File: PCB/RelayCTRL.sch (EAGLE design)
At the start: 20 parts, among them Q2 BC848 30V 100mA, Q3 IRLML6402, U1 SN74HC4066D

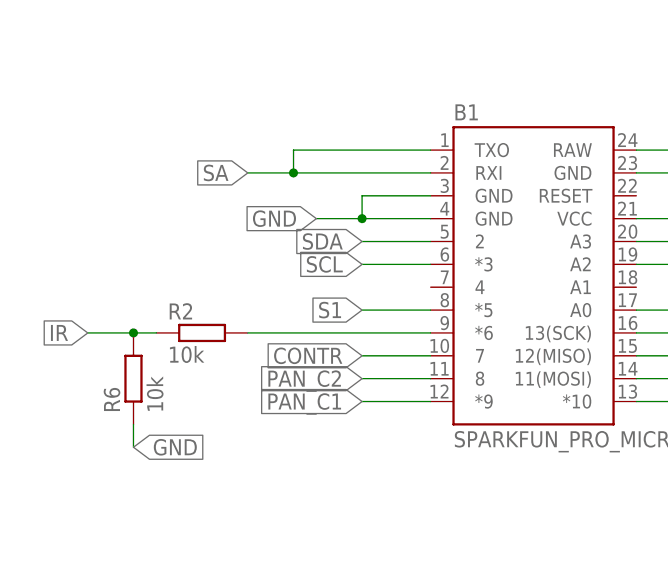
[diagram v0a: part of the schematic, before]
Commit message: fixed pcb error
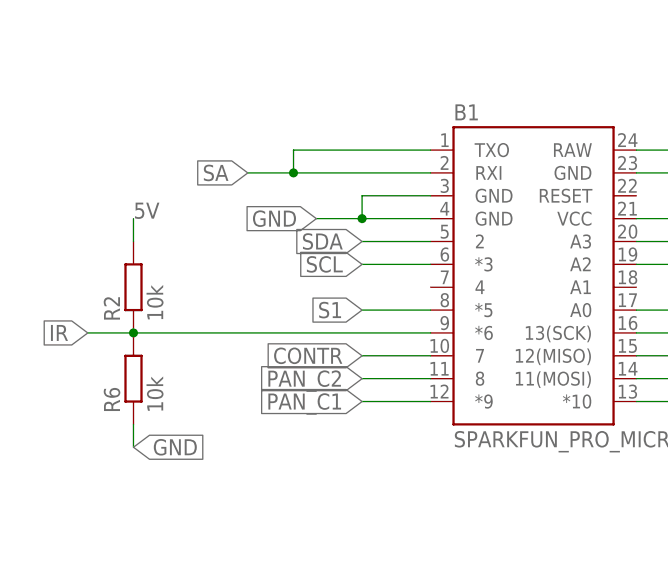
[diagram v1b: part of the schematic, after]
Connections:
- removed net N$1: B1.*6, R2.2
- net 5V: now also R2.2
- net IR: now also B1.*6
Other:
- moved on the sheet: R2
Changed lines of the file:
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@@
 <attribute name="TP_SIGNAL_NAME" x="95.25" y="-39.37" size="1.778" layer="97" rot="R180"/>
 </instance>
-<instance part="R2" gate="G$1" x="30.48" y="20.32" smashed="yes">
-<attribute name="NAME" x="26.67" y="21.8186" size="1.778" layer="95"/>
-<attribute name="VALUE" x="26.67" y="17.018" size="1.778" layer="96"/>
+<instance part="R2" gate="G$1" x="22.86" y="25.4" smashed="yes" rot="R90">
+<attribute name="NAME" x="21.3614" y="21.59" size="1.778" layer="95" rot="R90"/>
+<attribute name="VALUE" x="26.162" y="21.59" size="1.778" layer="96" rot="R90"/>
 </instance>
 <instance part="R6" gate="G$1" x="22.86" y="15.24" smashed="yes" rot="R90">
@@
 <wire x1="88.9" y1="-38.1" x2="88.9" y2="-33.02" width="0.1524" layer="91"/>
 <label x="88.9" y="-33.02" size="1.778" layer="95" rot="R90" xref="yes"/>
+</segment>
+<segment>
+<pinref part="R2" gate="G$1" pin="2"/>
+<wire x1="22.86" y1="30.48" x2="22.86" y2="33.02" width="0.1524" layer="91"/>
+<label x="22.86" y="33.02" size="1.778" layer="95"/>
 </segment>
 </net>
@@
 </segment>
 </net>
-<net name="N$1" class="0">
-<segment>
-<pinref part="B1" gate="G$1" pin="*6"/>
-<pinref part="R2" gate="G$1" pin="2"/>
-<wire x1="55.88" y1="20.32" x2="35.56" y2="20.32" width="0.1524" layer="91"/>
-</segment>
-</net>
 <net name="3V" class="0">
 <segment>
@@
 <segment>
 <pinref part="R2" gate="G$1" pin="1"/>
-<wire x1="25.4" y1="20.32" x2="22.86" y2="20.32" width="0.1524" layer="91"/>
 <label x="17.78" y="20.32" size="1.778" layer="95" rot="R180" xref="yes"/>
 <pinref part="R6" gate="G$1" pin="2"/>
 <wire x1="22.86" y1="20.32" x2="17.78" y2="20.32" width="0.1524" layer="91"/>
 <junction x="22.86" y="20.32"/>
-</segment>
-<segment>
+<pinref part="B1" gate="G$1" pin="*6"/>
+<wire x1="22.86" y1="20.32" x2="55.88" y2="20.32" width="0.1524" layer="91"/>
+</segment>
+<segment>
